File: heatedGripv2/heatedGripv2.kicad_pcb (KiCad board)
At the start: 2 copper layers, 32.3 x 16.5 mm, 23 parts, among them J1 TEMP, J2 HEAT, J3 BATT, J4 USB_C_Receptacle_PowerOnly_6P, J5 PROG, Q1 DMN3300U, SW1 SW_Push, U1 ATtiny204-SS, U2 MCP73811T-420I-OT, U3 REG710NA-3.3/3K

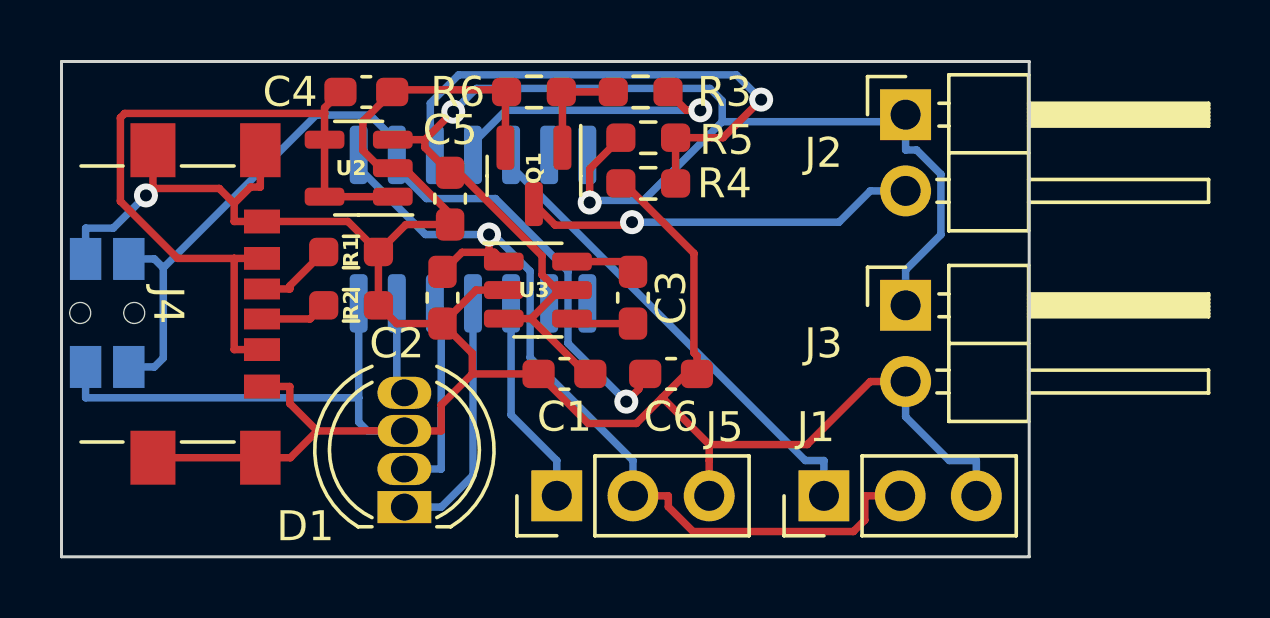
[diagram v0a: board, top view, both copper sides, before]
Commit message: Added v3
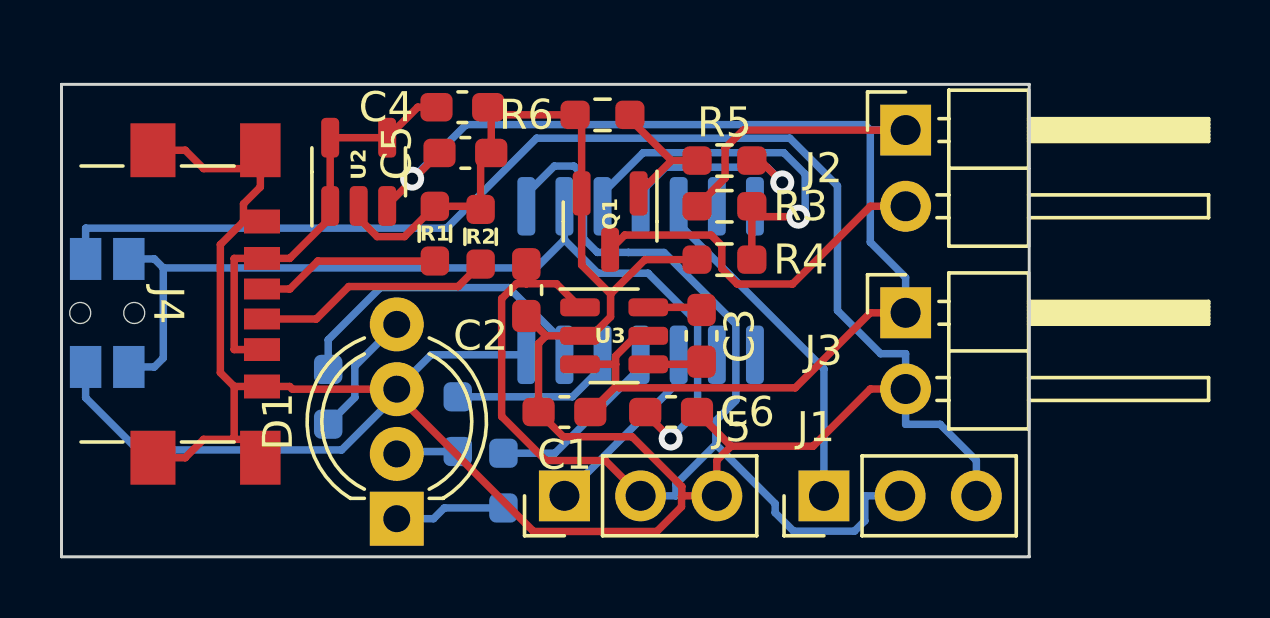
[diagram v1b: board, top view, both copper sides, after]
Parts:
- added R7: 55, Resistor_SMD:R_0603_1608Metric_Pad0.98x0.95mm_HandSolder, B.Cu at (132.3, 101.9)
- added R8: 5, Resistor_SMD:R_0603_1608Metric_Pad0.98x0.95mm_HandSolder, B.Cu at (130.8, 100.0)
- added R9: 5, Resistor_SMD:R_0603_1608Metric_Pad0.98x0.95mm_HandSolder, B.Cu at (126.5, 99.1)
- D1: footprint LED_THT:LED_D5.0mm-4_RGB -> LED_THT:LED_D5.0mm-4_RGB_Wide_Pins
- Q1: value DMN3300U -> DMN2024U-7
- moved U1 5.84 mm to (136.9, 95.2)
- moved R2 4.89 mm to (131.6, 93.7), turned to 90 degrees
- moved R5 3.61 mm to (139.7, 91.2)
- moved R4 3.59 mm to (139.7, 94.5)
- moved R3 3.42 mm to (139.7, 92.7)
- moved C4 3.24 mm to (131.0, 89.4)
- moved U3 2.96 mm to (136.0, 97.0)
- moved Q1 2.96 mm to (135.9, 93.2)
- moved R1 2.86 mm to (130.0, 93.6), turned to 90 degrees
- moved C2 2.81 mm to (133.1, 95.5)
- moved C3 2.62 mm to (138.9, 97.0)
- moved R6 2.41 mm to (135.6, 89.7)
- moved C5 1.61 mm to (131.1, 90.9), turned to 0 degrees
- moved C1 1.27 mm to (134.4, 99.6)
- moved C6 1.27 mm to (137.9, 99.6)
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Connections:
- D1 pad 1: /LED0 -> Net-(D1-RK)
- D1 pad 2: /LED1 -> Net-(D1-GK)
- D1 pad 4: /LED2 -> Net-(D1-BK)
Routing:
- net GND: track 103.7 -> 141.7 mm, vias 1 -> 0
- net +3.3V: track 30.1 -> 40.9 mm, vias 1 -> 0
- net VBUS: track 25.1 -> 14.4 mm
- net /LED2: track 3.09 -> 10.7 mm
- net Net-(J4-CC2): track 2.24 -> 8.04 mm
- net /BAT_VOLT: track 18.4 -> 12.9 mm
- net /TEMP: track 16.0 -> 11.7 mm
- net Net-(D1-BK): track 0.00 -> 4.27 mm
- net Net-(D1-RK): track 0.00 -> 3.70 mm
- net Net-(J4-CC1): track 2.63 -> 6.15 mm
- net +BATT: track 47.0 -> 50.5 mm, vias 2 -> 1
- net /GATE: track 9.75 -> 7.06 mm
- net /LED0: track 8.46 -> 6.18 mm
- net Net-(D1-GK): track 0.00 -> 2.07 mm
- net /BUTTON: track 30.1 -> 31.5 mm
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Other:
- board size 32.3 x 16.5 mm -> 32.3 x 15.7 mm
